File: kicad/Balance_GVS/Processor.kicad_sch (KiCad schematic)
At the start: 26 parts, among them SW3 SW_Push, SW4 SW_Push, U1 ESP32-WROOM-32E, U10 INA219BxD, U2 ESP32-WROOM-32E-N4, U9 MCP4725xxx-xCH

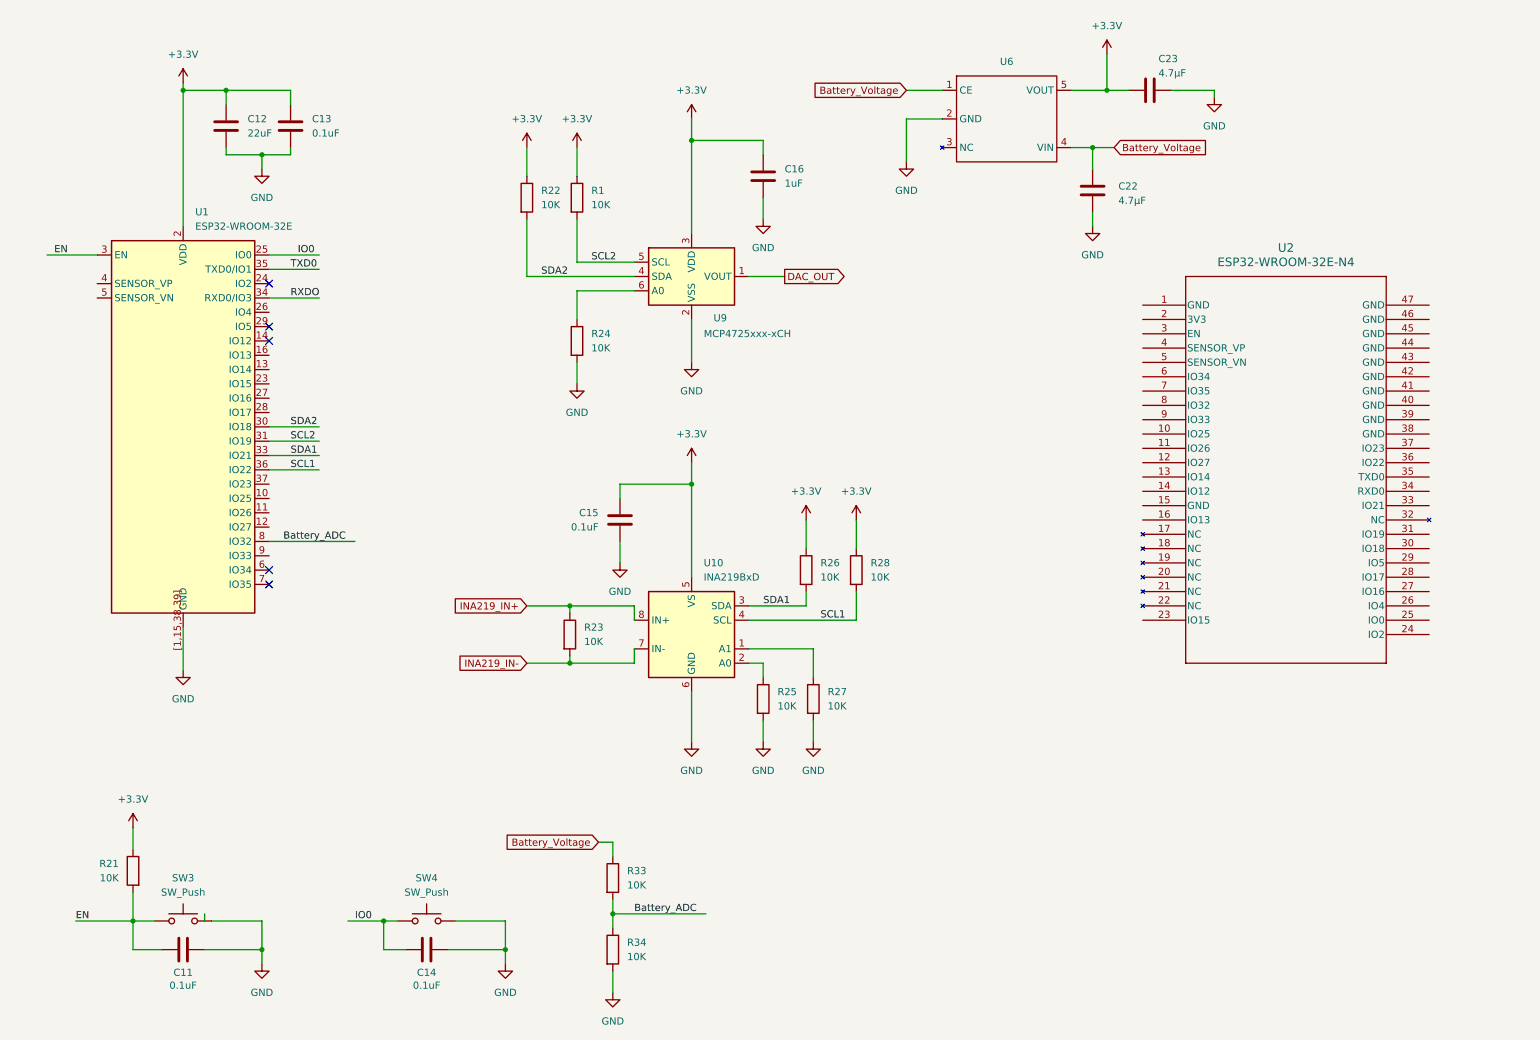
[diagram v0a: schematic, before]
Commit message: Add Processor User IO
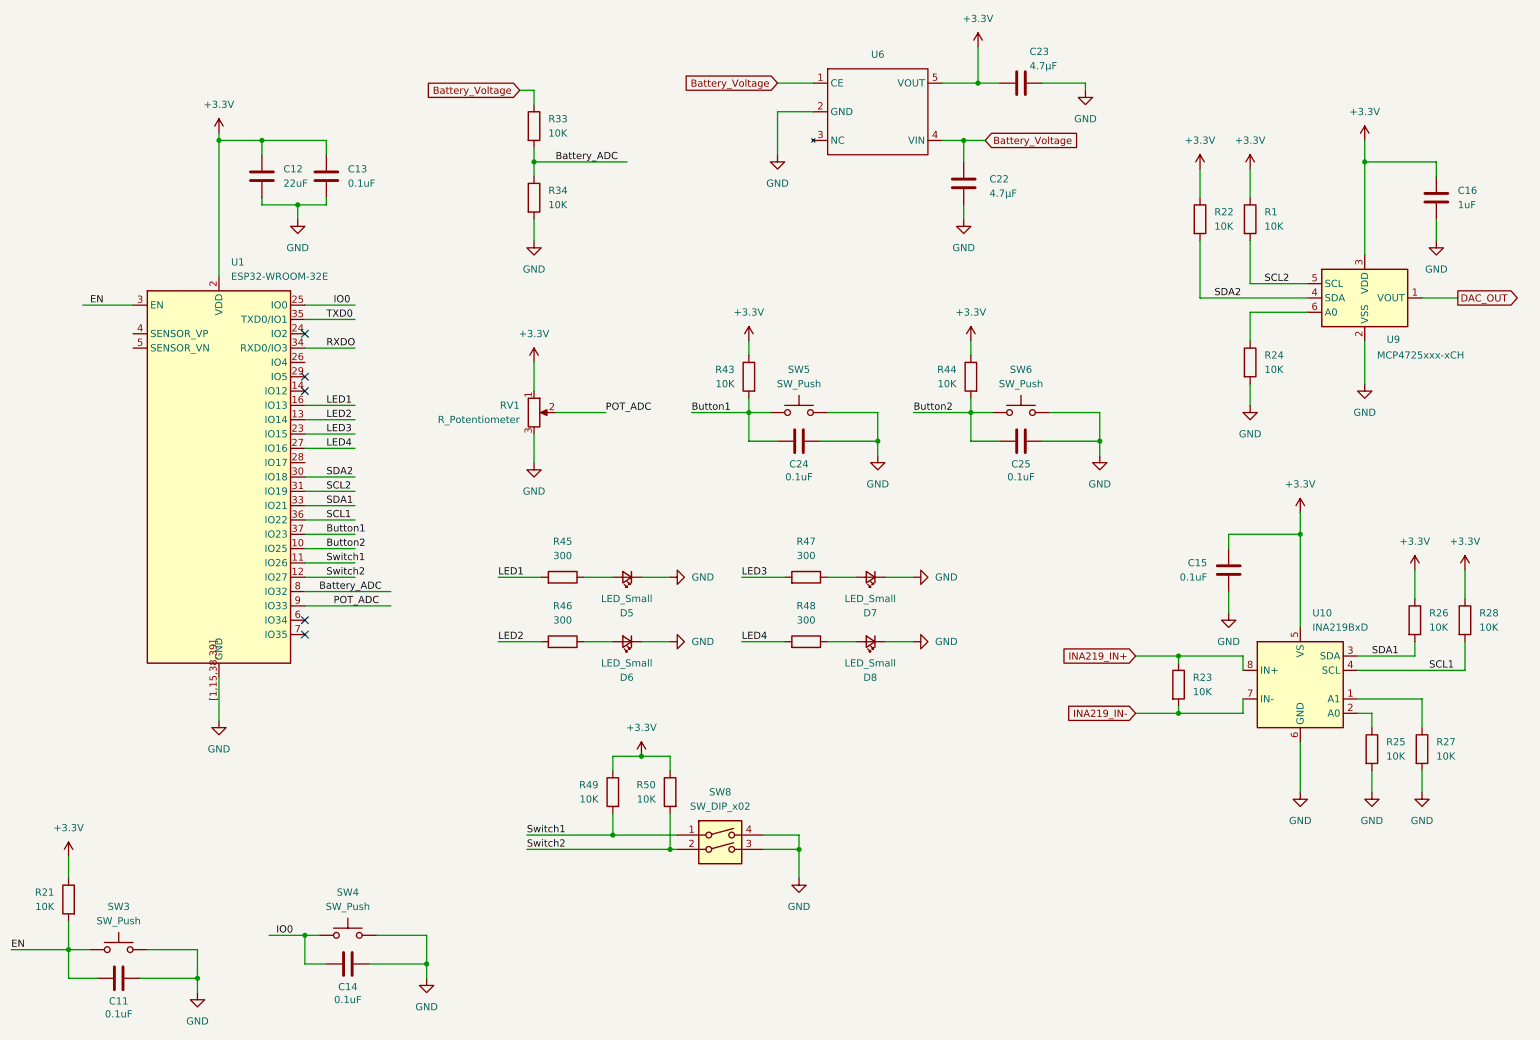
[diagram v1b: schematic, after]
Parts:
- removed U2: ESP32-WROOM-32E-N4, ESP32-WROOM_32E_N4_footprints:ESP32­WROOM­32E_EXP, symbol ESP32-WROOM_32E_N4:ESP32-WROOM-32E-N4
- added C24, C25: 0.1uF, RF_Converter:Balun_Johanson_0900PC15J0013, symbol Device:C
- added D5, D6, D7, D8: LED_Small, symbol Device:LED_Small
- added R43, R44, R49, R50: 10K, symbol Device:R
- added R45, R46, R47, R48: 300, symbol Device:R
- added RV1: R_Potentiometer, Package_SO:TSSOP-20_4.4x6.5mm_P0.65mm, symbol Device:R_Potentiometer
- added SW5, SW6: SW_Push, RF_Module:ESP32-WROOM-32E, symbol Switch:SW_Push
- added SW8: SW_DIP_x02, symbol Switch:SW_DIP_x02
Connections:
- net +3.3V: now also R43.1, R44.1, R49.1, R50.1, RV1.1
- net GND: now also C24.2, C25.2, D5.1 (K), D6.1 (K), D7.1 (K), D8.1 (K), RV1.3, SW5.1, SW6.1, SW8.3, SW8.4
- net Button2: now reaches U1.10 (IO25)
- net Button2: now also C25.1, R44.2, SW6.2
- net Switch1: now reaches U1.11 (IO26)
- net Switch1: now also R49.2, SW8.1
- net Switch2: now reaches U1.12 (IO27)
- net Switch2: now also R50.2, SW8.2
- net LED2: now reaches U1.13 (IO14)
- net LED2: now also R46.2
- net LED1: now reaches U1.16 (IO13)
- net LED1: now also R45.2
- net LED3: now reaches U1.23 (IO15)
- net LED3: now also R47.2
- net LED4: now reaches U1.27 (IO16)
- net LED4: now also R48.2
- net Button1: now reaches U1.37 (IO23)
- net Button1: now also C24.1, R43.2, SW5.2
- net POT_ADC: now reaches U1.9 (IO33)
- net POT_ADC: now also RV1.2
- new net: D8.2 (A), R48.1
- new net: D5.2 (A), R45.1
- new net: D7.2 (A), R47.1
- new net: D6.2 (A), R46.1
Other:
- moved on the sheet: C11, C12, C13, C14, C15, C16, C22, C23, R1, R21, R22, R23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
